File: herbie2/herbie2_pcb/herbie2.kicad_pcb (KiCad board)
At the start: 2 copper layers, 146.1 x 100.3 mm, 6 parts

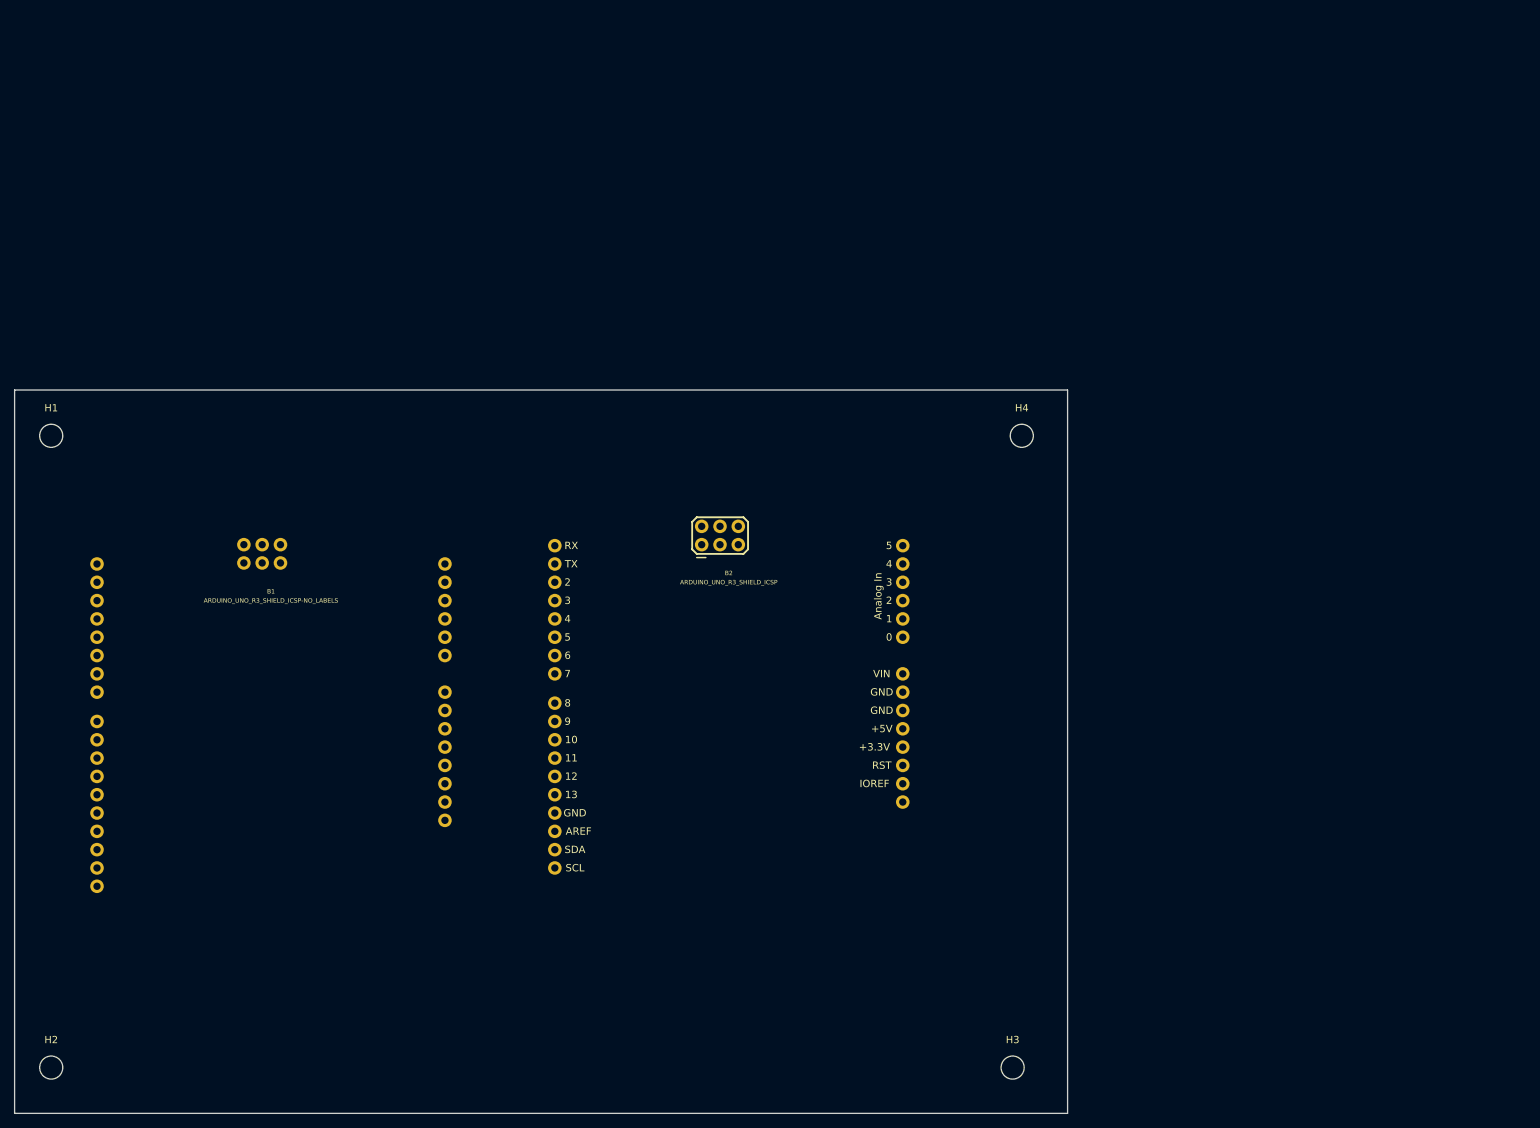
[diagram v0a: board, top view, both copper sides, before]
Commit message: updated PCB
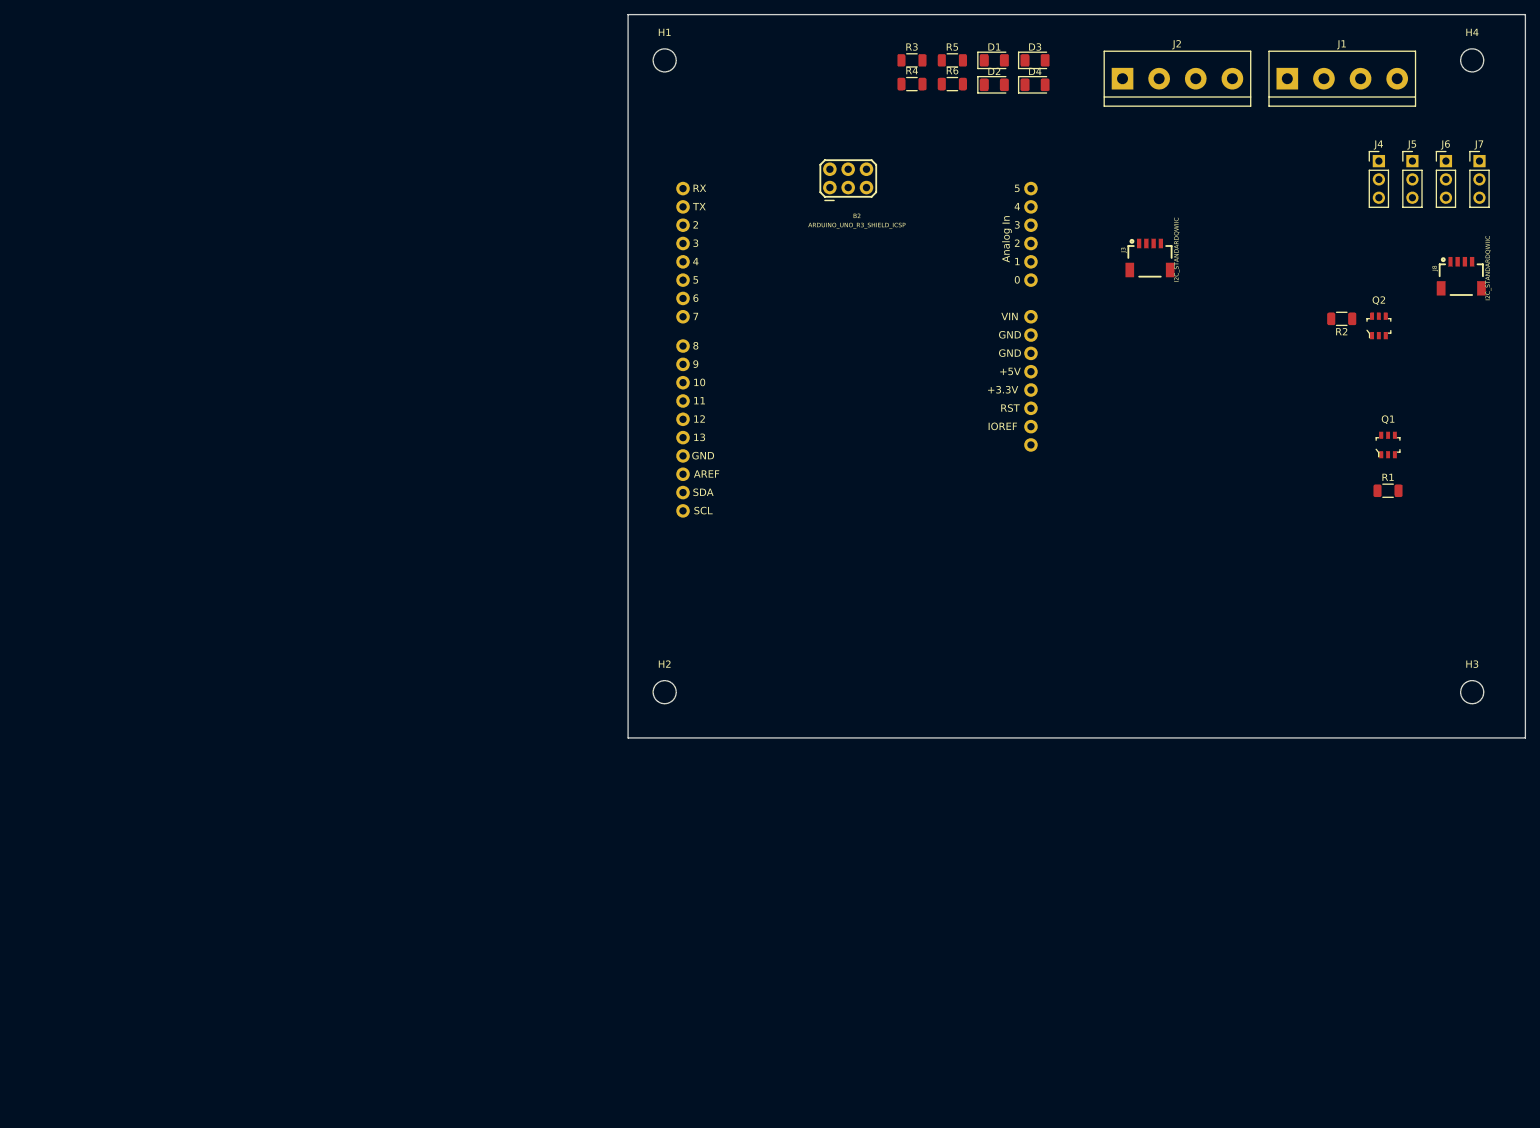
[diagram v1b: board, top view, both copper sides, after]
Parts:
- removed B1: ARDUINO_UNO_R3_SHIELD_ICSP-NO_LABELS, Sparkfun_boards:UNO_R3_SHIELD_ICSP_NOLABELS
- added D1: LED, LED_SMD:LED_1206_3216Metric, F.Cu at (152.4, 44.5)
- added D2: LED, LED_SMD:LED_1206_3216Metric, F.Cu at (152.4, 47.8)
- added D3: LED, LED_SMD:LED_1206_3216Metric, F.Cu at (158.1, 44.5)
- added D4: LED, LED_SMD:LED_1206_3216Metric, F.Cu at (158.1, 47.8)
- added J1: Screw_Terminal_01x04, TerminalBlock:TerminalBlock_bornier-4_P5.08mm, F.Cu at (193.0, 47.0)
- added J2: Screw_Terminal_01x04, TerminalBlock:TerminalBlock_bornier-4_P5.08mm, F.Cu at (170.2, 47.0)
- added J3: I2C_STANDARDQWIIC, Connectors:1X04_1MM_RA, F.Cu at (174.0, 69.8)
- added J4: Servo0, Connector_PinHeader_2.54mm:PinHeader_1x03_P2.54mm_Vertical, F.Cu at (205.7, 58.4)
- added J5: Servo1, Connector_PinHeader_2.54mm:PinHeader_1x03_P2.54mm_Vertical, F.Cu at (210.4, 58.4)
- added J6: Servo2, Connector_PinHeader_2.54mm:PinHeader_1x03_P2.54mm_Vertical, F.Cu at (215.0, 58.4)
- added J7: Servo3, Connector_PinHeader_2.54mm:PinHeader_1x03_P2.54mm_Vertical, F.Cu at (219.7, 58.4)
- added J8: I2C_STANDARDQWIIC, Connectors:1X04_1MM_RA, F.Cu at (217.2, 72.4)
- added Q1: LTC4412ES6_TRMPBF, digikey-footprints:SOT-23-6, F.Cu at (207.0, 97.8)
- added Q2: LTC4412ES6_TRMPBF, digikey-footprints:SOT-23-6, F.Cu at (205.7, 81.3)
- added R1: 470K, Resistor_SMD:R_1206_3216Metric, F.Cu at (207.0, 104.1)
- added R2: 470K, Resistor_SMD:R_1206_3216Metric, F.Cu at (200.6, 80.3)
- added R3: R, Resistor_SMD:R_1206_3216Metric, F.Cu at (141.0, 44.5)
- added R4: R, Resistor_SMD:R_1206_3216Metric, F.Cu at (141.0, 47.7)
- added R5: R, Resistor_SMD:R_1206_3216Metric, F.Cu at (146.6, 44.5)
- added R6: R, Resistor_SMD:R_1206_3216Metric, F.Cu at (146.6, 47.7)
- moved H1 99.8 mm to (106.7, 44.5)
- moved H2 99.8 mm to (106.7, 132.1)
- moved H3 82.3 mm to (218.7, 132.1)
- moved H4 81.3 mm to (218.7, 44.5)
- moved B2 52.6 mm to (133.3, 86.4)
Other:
- board size 146.1 x 100.3 mm -> 124.5 x 100.3 mm
